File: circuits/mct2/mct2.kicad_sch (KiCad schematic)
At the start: 15 parts

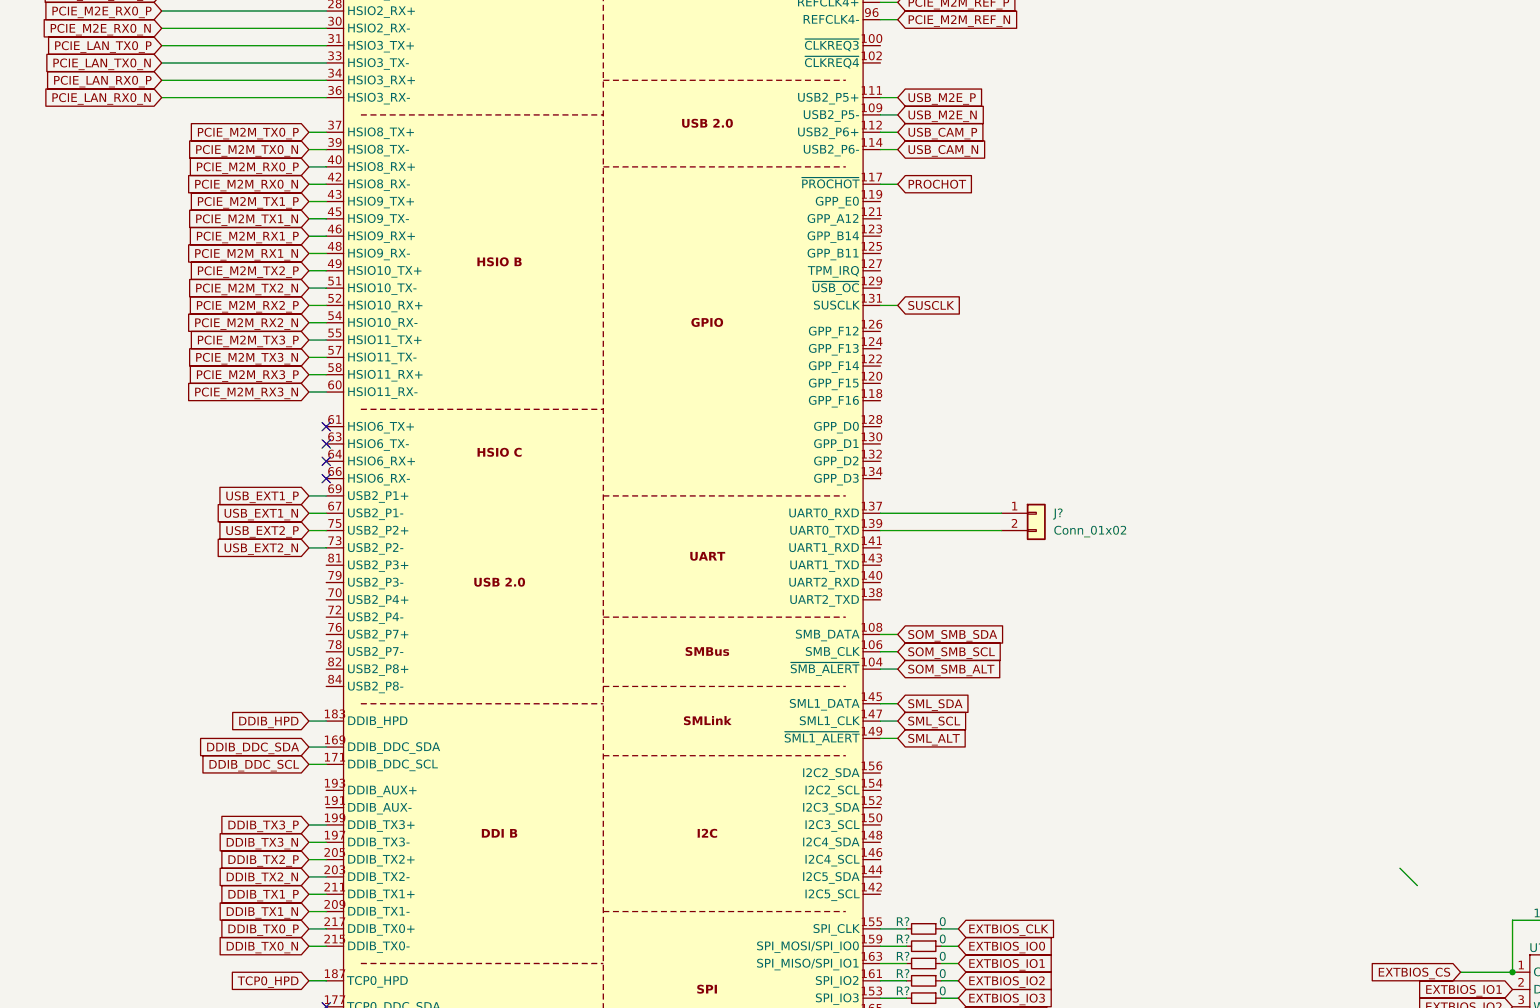
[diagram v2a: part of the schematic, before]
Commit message: Aug 19, 2024
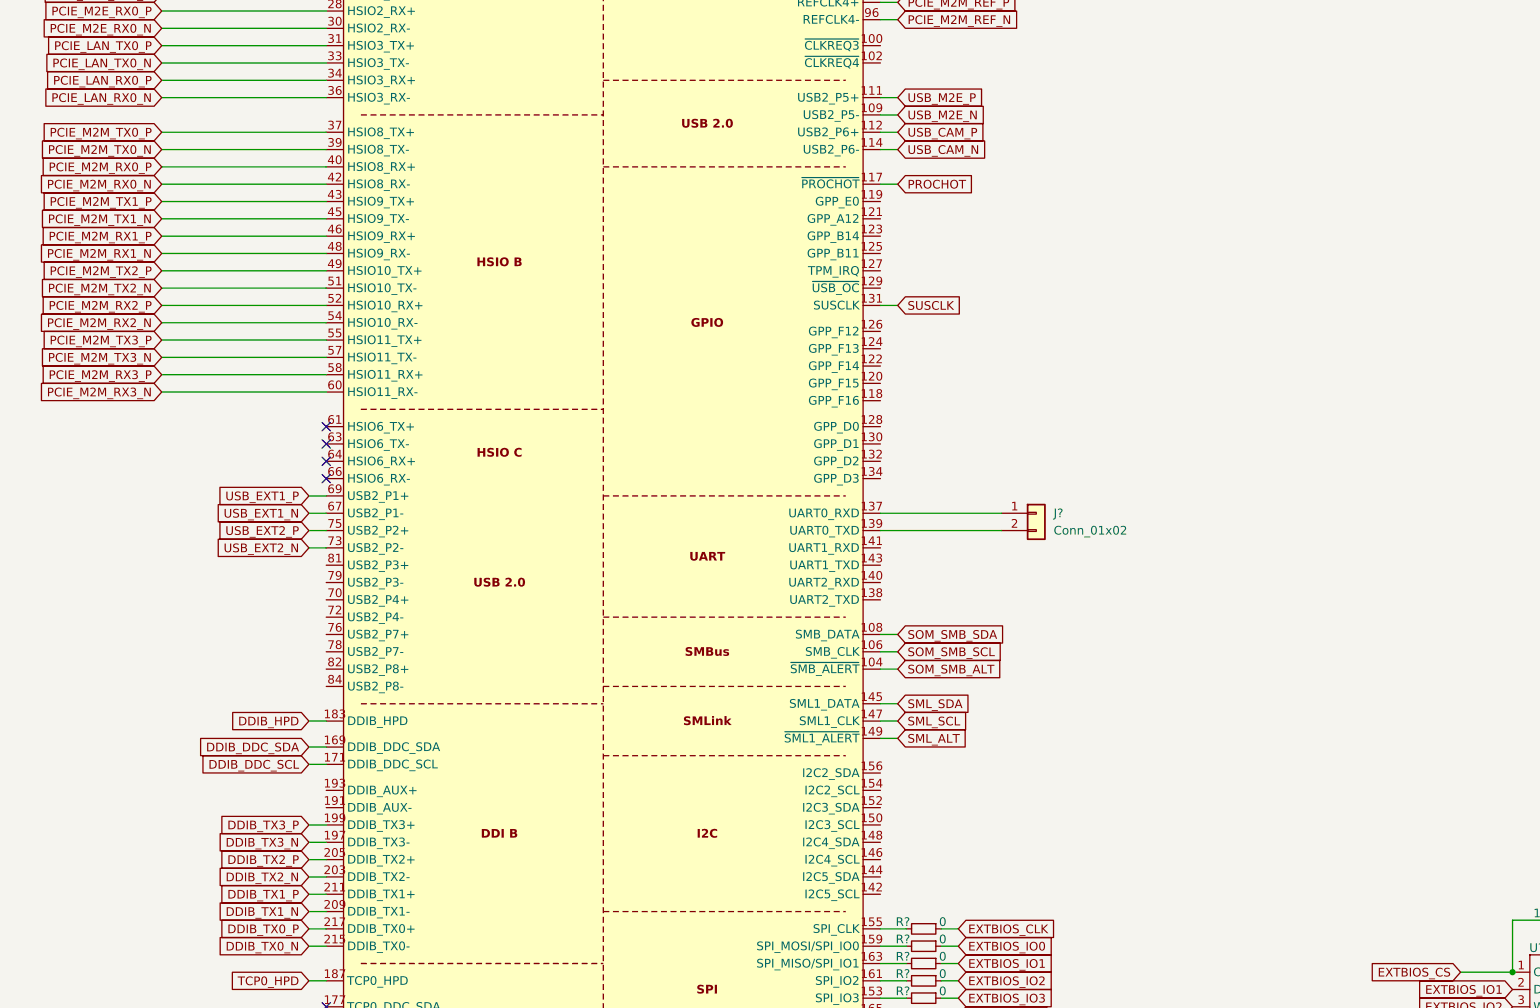
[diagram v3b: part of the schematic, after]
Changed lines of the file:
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@@
 		(at 501.65 537.21)
 	)
-	(bus_entry
-		(at 659.13 516.89)
-		(size 2.54 2.54)
-		(stroke
-			(width 0)
-			(type default)
-		)
-	)
 	(wire
 		(pts
@@
 	(wire
 		(pts
-			(xy 499.11 414.02) (xy 501.65 414.02)
+			(xy 477.52 414.02) (xy 501.65 414.02)
 		)
 		(stroke
@@
 	(wire
 		(pts
-			(xy 499.11 411.48) (xy 501.65 411.48)
+			(xy 477.52 411.48) (xy 501.65 411.48)
 		)
 		(stroke
@@
 	(wire
 		(pts
-			(xy 499.11 408.94) (xy 501.65 408.94)
+			(xy 477.52 408.94) (xy 501.65 408.94)
 		)
 		(stroke
@@
 	(wire
 		(pts
-			(xy 499.11 419.1) (xy 501.65 419.1)
+			(xy 477.52 419.1) (xy 501.65 419.1)
 		)
 		(stroke
@@
 	(wire
 		(pts
-			(xy 499.11 431.8) (xy 501.65 431.8)
+			(xy 477.52 431.8) (xy 501.65 431.8)
 		)
 		(stroke
@@
 	(wire
 		(pts
-			(xy 499.11 416.56) (xy 501.65 416.56)
+			(xy 477.52 416.56) (xy 501.65 416.56)
 		)
 		(stroke
@@
 	(wire
 		(pts
-			(xy 499.11 424.18) (xy 501.65 424.18)
+			(xy 477.52 424.18) (xy 501.65 424.18)
 		)
 		(stroke
@@
 	(wire
 		(pts
-			(xy 499.11 439.42) (xy 501.65 439.42)
+			(xy 477.52 439.42) (xy 501.65 439.42)
 		)
 		(stroke
@@
 	(wire
 		(pts
-			(xy 499.11 444.5) (xy 501.65 444.5)
+			(xy 477.52 444.5) (xy 501.65 444.5)
 		)
 		(stroke
@@
 	(wire
 		(pts
-			(xy 499.11 421.64) (xy 501.65 421.64)
+			(xy 477.52 421.64) (xy 501.65 421.64)
 		)
 		(stroke
@@
 	(wire
 		(pts
-			(xy 499.11 447.04) (xy 501.65 447.04)
+			(xy 477.52 447.04) (xy 501.65 447.04)
 		)
 		(stroke
@@
 	(wire
 		(pts
-			(xy 499.11 426.72) (xy 501.65 426.72)
+			(xy 477.52 426.72) (xy 501.65 426.72)
 		)
 		(stroke
@@
 	(wire
 		(pts
-			(xy 499.11 441.96) (xy 501.65 441.96)
+			(xy 477.52 441.96) (xy 501.65 441.96)
 		)
 		(stroke
@@
 	(wire
 		(pts
-			(xy 499.11 434.34) (xy 501.65 434.34)
+			(xy 477.52 434.34) (xy 501.65 434.34)
 		)
 		(stroke
@@
 	(wire
 		(pts
-			(xy 499.11 429.26) (xy 501.65 429.26)
+			(xy 477.52 429.26) (xy 501.65 429.26)
 		)
 		(stroke
@@
 	(wire
 		(pts
-			(xy 499.11 436.88) (xy 501.65 436.88)
+			(xy 477.52 436.88) (xy 501.65 436.88)
 		)
 		(stroke
@@
 	(global_label "PCIE_M2M_TX0_P"
 		(shape input)
-		(at 499.11 408.94 180)
+		(at 477.52 408.94 180)
 		(fields_autoplaced yes)
 		(effects
@@
 		)
 		(property "Intersheetrefs" "${INTERSHEET_REFS}"
-			(at 479.2521 408.94 0)
+			(at 457.6621 408.94 0)
 			(effects
 				(font
@@
 	(global_label "PCIE_M2M_RX1_N"
 		(shape input)
-		(at 499.11 426.72 180)
+		(at 477.52 426.72 180)
 		(fields_autoplaced yes)
 		(effects
@@
 		)
 		(property "Intersheetrefs" "${INTERSHEET_REFS}"
-			(at 478.8892 426.72 0)
+			(at 457.2992 426.72 0)
 			(effects
 				(font
@@
 	(global_label "PCIE_M2M_TX0_N"
 		(shape input)
-		(at 499.11 411.48 180)
+		(at 477.52 411.48 180)
 		(fields_autoplaced yes)
 		(effects
@@
 		)
 		(property "Intersheetrefs" "${INTERSHEET_REFS}"
-			(at 479.1916 411.48 0)
+			(at 457.6016 411.48 0)
 			(effects
 				(font
@@
 	(global_label "PCIE_M2M_RX3_N"
 		(shape input)
-		(at 499.11 447.04 180)
+		(at 477.52 447.04 180)
 		(fields_autoplaced yes)
 		(effects
@@
 		)
 		(property "Intersheetrefs" "${INTERSHEET_REFS}"
-			(at 478.8892 447.04 0)
+			(at 457.2992 447.04 0)
 			(effects
 				(font
@@
 	(global_label "PCIE_M2M_RX2_N"
 		(shape input)
-		(at 499.11 436.88 180)
+		(at 477.52 436.88 180)
 		(fields_autoplaced yes)
 		(effects
@@
 		)
 		(property "Intersheetrefs" "${INTERSHEET_REFS}"
-			(at 478.8892 436.88 0)
+			(at 457.2992 436.88 0)
 			(effects
 				(font
@@
 	(global_label "PCIE_M2M_TX3_N"
 		(shape input)
-		(at 499.11 441.96 180)
+		(at 477.52 441.96 180)
 		(fields_autoplaced yes)
 		(effects
@@
 		)
 		(property "Intersheetrefs" "${INTERSHEET_REFS}"
-			(at 479.1916 441.96 0)
+			(at 457.6016 441.96 0)
 			(effects
 				(font
@@
 	(global_label "PCIE_M2M_TX1_N"
 		(shape input)
-		(at 499.11 421.64 180)
+		(at 477.52 421.64 180)
 		(fields_autoplaced yes)
 		(effects
@@
 		)
 		(property "Intersheetrefs" "${INTERSHEET_REFS}"
-			(at 479.1916 421.64 0)
+			(at 457.6016 421.64 0)
 			(effects
 				(font
@@
 	(global_label "PCIE_M2M_TX2_N"
 		(shape input)
-		(at 499.11 431.8 180)
+		(at 477.52 431.8 180)
 		(fields_autoplaced yes)
 		(effects
@@
 		)
 		(property "Intersheetrefs" "${INTERSHEET_REFS}"
-			(at 479.1916 431.8 0)
+			(at 457.6016 431.8 0)
 			(effects
 				(font
@@
 	(global_label "PCIE_M2M_RX0_P"
 		(shape input)
-		(at 499.11 414.02 180)
+		(at 477.52 414.02 180)
 		(fields_autoplaced yes)
 		(effects
@@
 		)
 		(property "Intersheetrefs" "${INTERSHEET_REFS}"
-			(at 478.9497 414.02 0)
+			(at 457.3597 414.02 0)
 			(effects
 				(font
@@
 	(global_label "PCIE_M2M_RX2_P"
 		(shape input)
-		(at 499.11 434.34 180)
+		(at 477.52 434.34 180)
 		(fields_autoplaced yes)
 		(effects
@@
 		)
 		(property "Intersheetrefs" "${INTERSHEET_REFS}"
-			(at 478.9497 434.34 0)
+			(at 457.3597 434.34 0)
 			(effects
 				(font
@@
 	(global_label "PCIE_M2M_RX3_P"
 		(shape input)
-		(at 499.11 444.5 180)
+		(at 477.52 444.5 180)
 		(fields_autoplaced yes)
 		(effects
@@
 		)
 		(property "Intersheetrefs" "${INTERSHEET_REFS}"
-			(at 478.9497 444.5 0)
+			(at 457.3597 444.5 0)
 			(effects
 				(font
@@
 	(global_label "PCIE_M2M_TX3_P"
 		(shape input)
-		(at 499.11 439.42 180)
+		(at 477.52 439.42 180)
 		(fields_autoplaced yes)
 		(effects
@@
 		)
 		(property "Intersheetrefs" "${INTERSHEET_REFS}"
-			(at 479.2521 439.42 0)
+			(at 457.6621 439.42 0)
 			(effects
 				(font
@@
 	(global_label "PCIE_M2M_RX0_N"
 		(shape input)
-		(at 499.11 416.56 180)
+		(at 477.52 416.56 180)
 		(fields_autoplaced yes)
 		(effects
@@
 		)
 		(property "Intersheetrefs" "${INTERSHEET_REFS}"
-			(at 478.8892 416.56 0)
+			(at 457.2992 416.56 0)
 			(effects
 				(font
@@
 	(global_label "PCIE_M2M_TX2_P"
 		(shape input)
-		(at 499.11 429.26 180)
+		(at 477.52 429.26 180)
 		(fields_autoplaced yes)
 		(effects
@@
 		)
 		(property "Intersheetrefs" "${INTERSHEET_REFS}"
-			(at 479.2521 429.26 0)
+			(at 457.6621 429.26 0)
 			(effects
 				(font
@@
 	(global_label "PCIE_M2M_RX1_P"
 		(shape input)
-		(at 499.11 424.18 180)
+		(at 477.52 424.18 180)
 		(fields_autoplaced yes)
 		(effects
@@
 		)
 		(property "Intersheetrefs" "${INTERSHEET_REFS}"
-			(at 478.9497 424.18 0)
+			(at 457.3597 424.18 0)
 			(effects
 				(font
@@
 	(global_label "PCIE_M2M_TX1_P"
 		(shape input)
-		(at 499.11 419.1 180)
+		(at 477.52 419.1 180)
 		(fields_autoplaced yes)
 		(effects
@@
 		)
 		(property "Intersheetrefs" "${INTERSHEET_REFS}"
-			(at 479.2521 419.1 0)
+			(at 457.6621 419.1 0)
 			(effects
 				(font
